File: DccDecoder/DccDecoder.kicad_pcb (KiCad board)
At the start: 2 copper layers, 116.8 x 35.6 mm, 27 parts, among them J14 +V, J15 M_OUT_B, J16 M_OUT_A, J17 GND, J3 0, J4 1, J5 2, J6 3, J8 DCC, Q1 T2N7002BK, Q2 T2N7002BK, Q3 T2N7002BK, Q4 T2N7002BK, Q5 T2N7002BK, SW1 SW_Push, U1 HT7533S, U2 BDR6133, U4 Pico

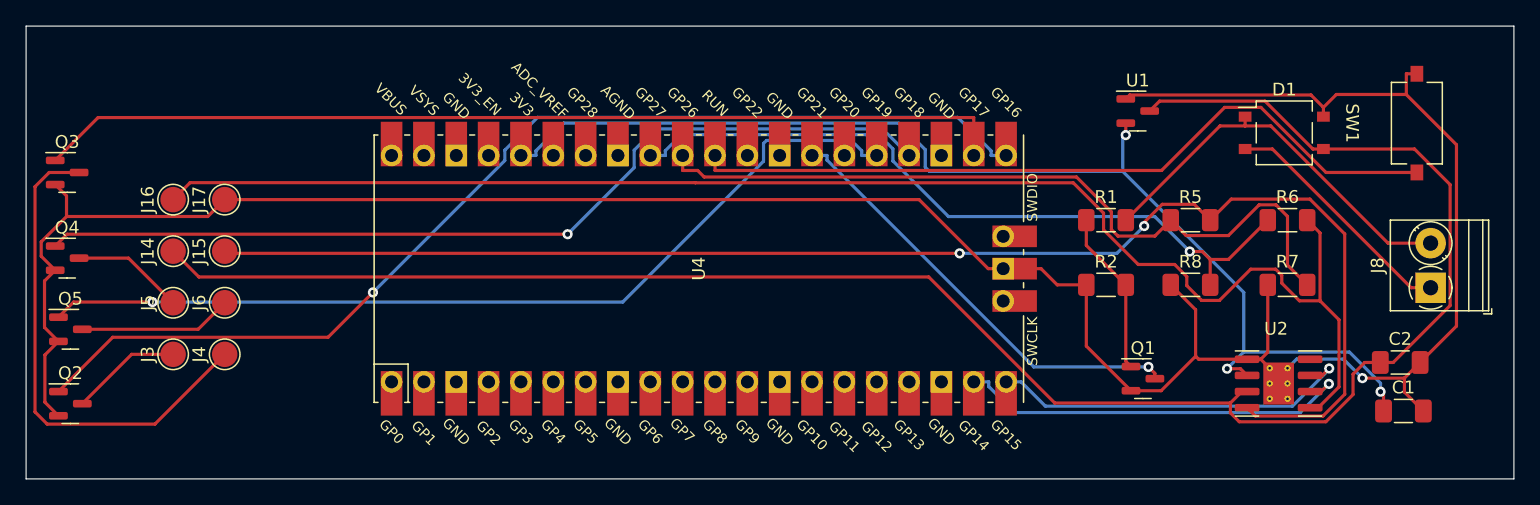
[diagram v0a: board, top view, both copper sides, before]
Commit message: 16:27 Arrakis.local
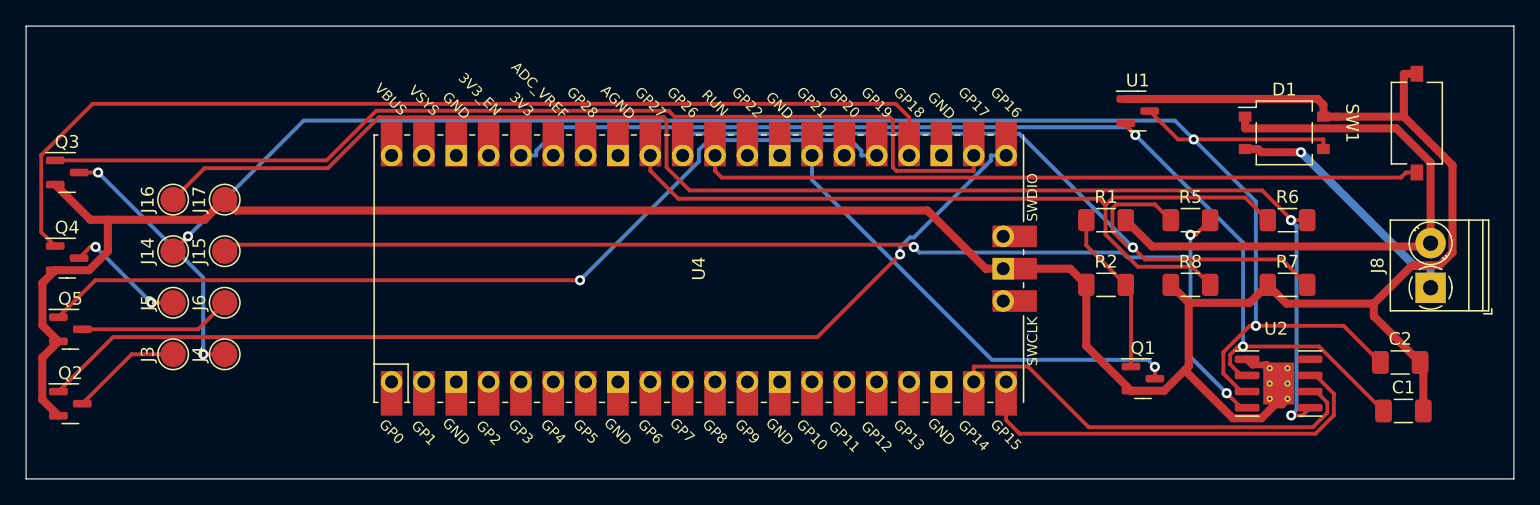
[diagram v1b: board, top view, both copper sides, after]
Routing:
- net /MOTOR_OUT_A: track 113.4 -> 94.2 mm, vias 2 -> 3
- net Net-(J4-Pin_1): track 39.2 -> 20.9 mm, vias 0 -> 2
- net Net-(J8-Pin_2): track 31.5 -> 47.8 mm
- net +V: track 148.8 -> 135.5 mm, vias 0 -> 3
- net GND: track 211.5 -> 220.1 mm, vias 1 -> 0
- net /GPIO18: track 72.5 -> 80.8 mm, vias 1 -> 0
- net /ADC_EMF_B: track 57.3 -> 64.0 mm, vias 1 -> 0
- net /GPIO15: track 29.2 -> 33.9 mm, vias 1 -> 0
- net /ADC_EMF_A: track 60.0 -> 64.5 mm, vias 0 -> 1
- net Net-(U4-RUN): track 60.5 -> 56.7 mm
- net +3V3: track 90.6 -> 87.9 mm, vias 3 -> 2
- net /GPIO16: track 85.3 -> 82.7 mm
- net /GPIO17: track 76.5 -> 79.1 mm
- net /GPIO14: track 31.8 -> 33.9 mm, vias 1 -> 0
- net /GPIO21: track 34.6 -> 35.9 mm
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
